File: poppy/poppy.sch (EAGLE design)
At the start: 7 parts, among them Q1 10MHz

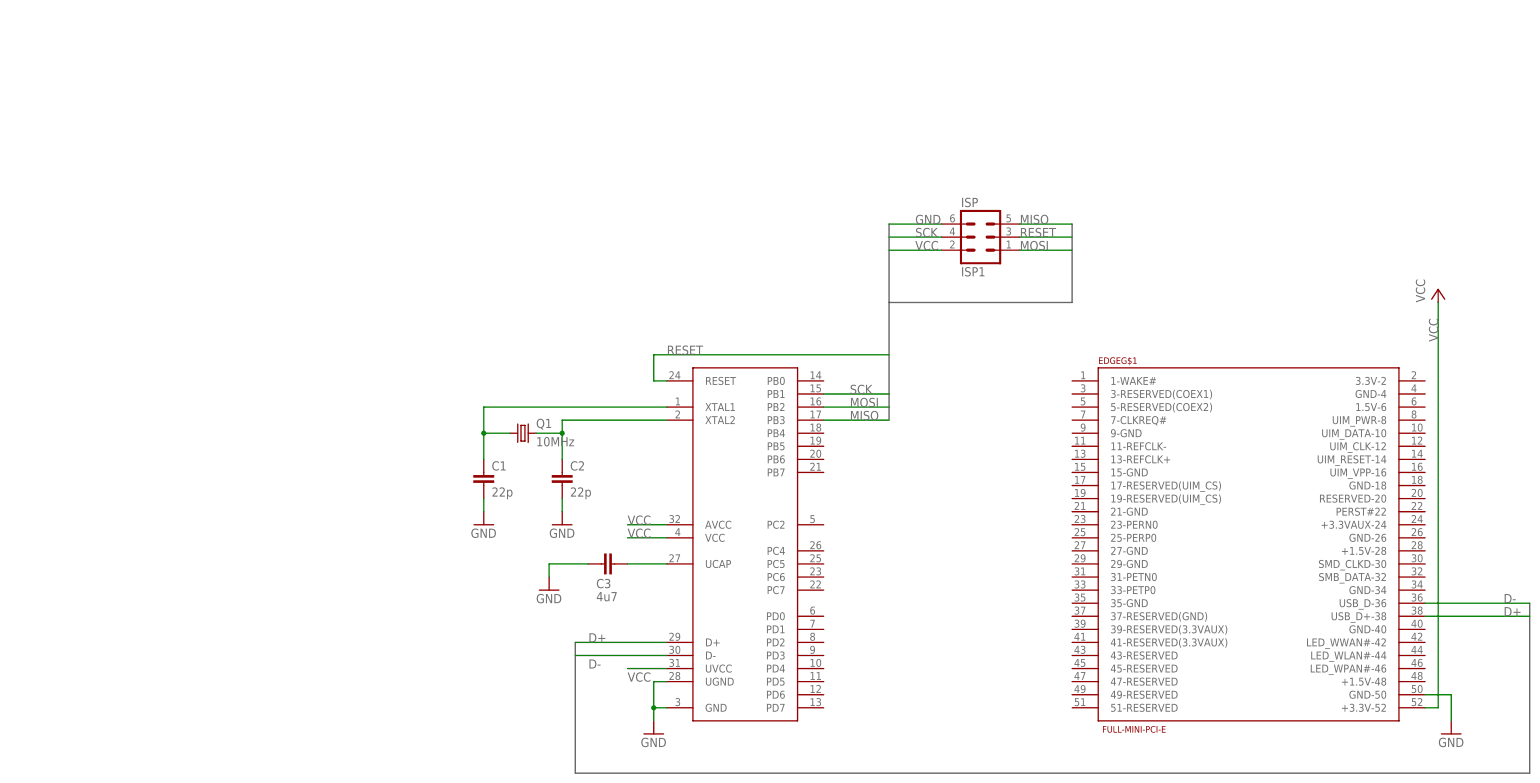
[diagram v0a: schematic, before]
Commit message: Routed
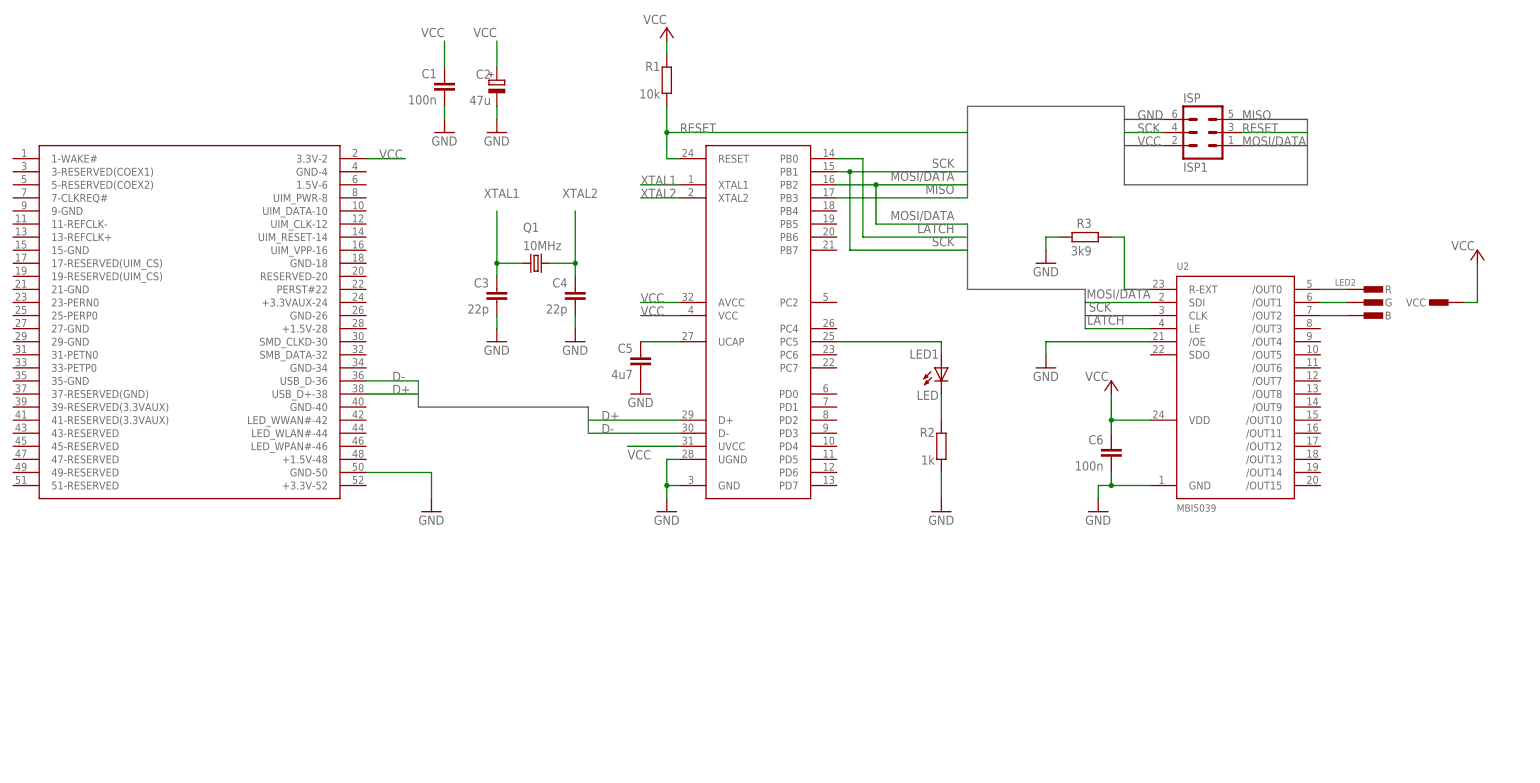
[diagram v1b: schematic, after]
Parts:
- removed U$1: AT90USB162, at90usb:AT90USB162
- added C4: 22p, resistor:C-EUC1206K
- added C5: 4u7, resistor:C-EUC1206K
- added C6: 100n, resistor:C-EUC1206K
- added LED1: LED, led:LEDCHIPLED_0805
- added LED2: CON-RGB-LED-EXT, _led-rgb:CON-RGB-LED-EXT
- added R1: 10k, resistor:R-EU_R1206
- added R2: 1k, resistor:R-EU_R1206
- added R3: 3k9, resistor:R-EU_R1206
- added U1: ATUSB, at90usb:AT90USB162
- added U2: MBI5039, _LedDrivers:MBI5039SOP24-300-1.00
- C1: value 22p -> 100n; device resistor:C-EUC1206K -> resistor:C-EUC4532
- C2: value 22p -> 47u; device resistor:C-EUC1206K -> resistor:CPOL-EU150CLZ-0810
- C3: value 4u7 -> 22p
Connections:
- removed net MOSI: ISP.1, U$1.PB2
- new net LATCH: U1.PB0, U2.LE
- new net MOSI/DATA: ISP.1, U1.PB2, U2.SDI
- new net N$3: LED2.R, U2./OUT0
- new net N$5: LED2.G, U2./OUT1
- new net N$6: LED2.B, U2./OUT2
- new net N$7: LED1.C, R2.2
- new net XTAL1: C3.1, Q1.1, U1.XTAL1
- new net XTAL2: C4.1, Q1.2, U1.XTAL2
- net D+: now also U1.D+; no longer U$1.D+
- net D-: now also U1.D-; no longer U$1.D-
- net GND: now also C2.-, C4.2, C5.2, C6.2, R2.1, R3.1, U1.GND, U1.UGND, U2./OE, U2.GND; no longer C2.2, U$1.GND, U$1.UGND
- net MISO: now also U1.PB3; no longer U$1.PB3
- net N$1: now also LED1.A, U1.PC5; no longer C2.1, Q1.2, U$1.XTAL2
- net N$2: now also R3.2, U2.R-EXT; no longer C1.1, Q1.1, U$1.XTAL1
- net N$4: now also C5.1, U1.UCAP; no longer C3.1, U$1.UCAP
- net RESET: now also R1.1, U1.RESET; no longer U$1.RESET
- net SCK: now also U1.PB1, U2.CLK; no longer U$1.PB1
- net VCC: now also C1.1, C2.+, C6.1, EDGEG$1.3.3V-2, LED2.VCC, R1.2, U1.AVCC, U1.UVCC, U1.VCC, U2.VDD; no longer EDGEG$1.+3.3V-52, U$1.AVCC, U$1.UVCC, U$1.VCC
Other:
- moved on the sheet: C1, C3, ISP, Q1
